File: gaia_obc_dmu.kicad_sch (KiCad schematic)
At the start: 7 parts, among them J2 Micro_SD_Card_Det2, U7 WLR089U0-I_RM

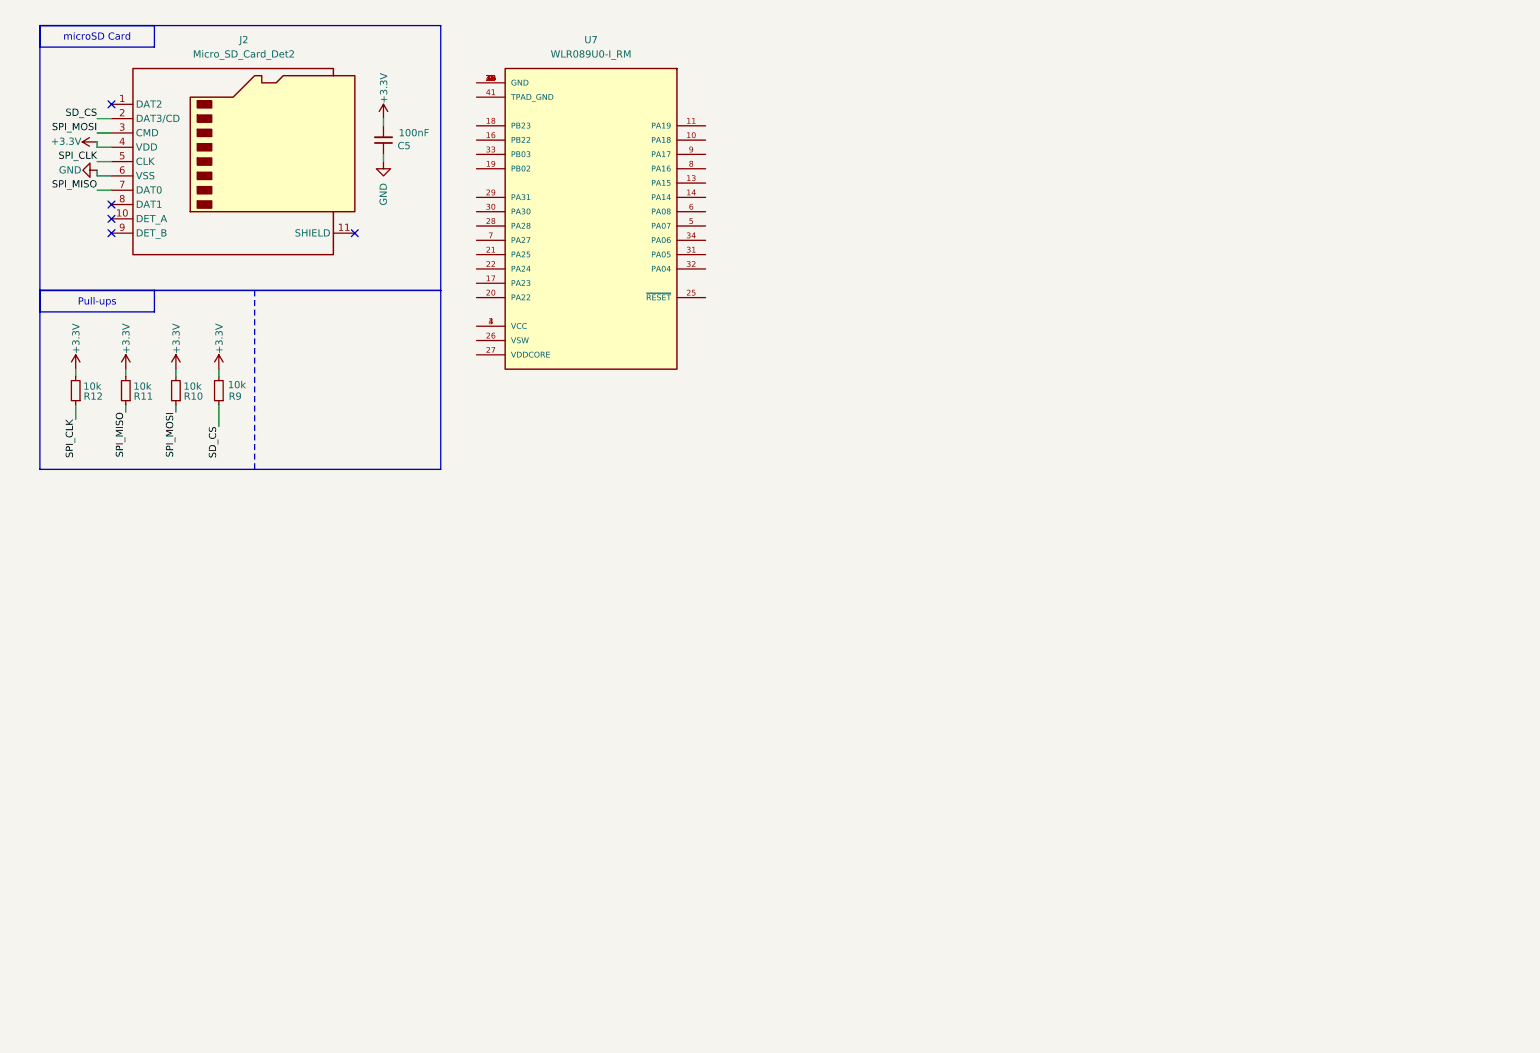
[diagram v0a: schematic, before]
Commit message: almost final release
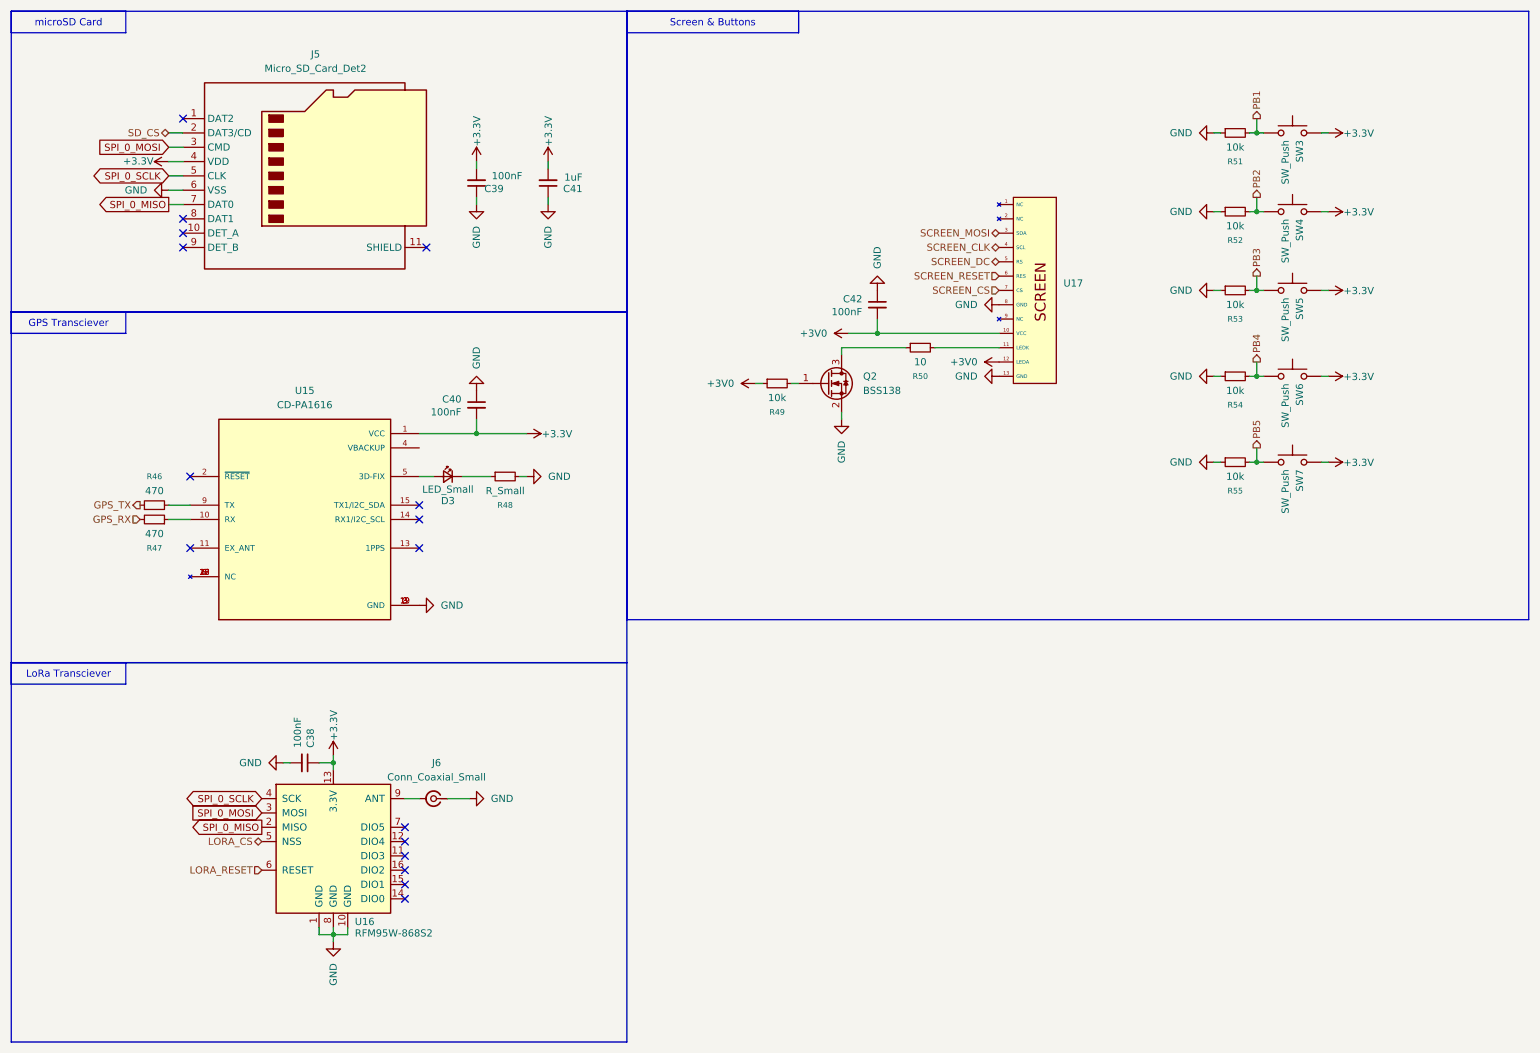
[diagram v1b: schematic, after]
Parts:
- removed R10, R11, R12, R9: 10k, symbol Device:R_Small
- removed U7: WLR089U0-I_RM, OnionSAT_Gaia:MODULE_WLR089U0-I_RM, symbol cs25_onionsat:WLR089U0-I_RM
- added C38, C40, C42: 100nF, Capacitor_SMD:C_0402_1005Metric, symbol Device:C_Small
- added C41: 1uF, Capacitor_SMD:C_0402_1005Metric, symbol Device:C_Small
- added D3: LED_Small, symbol Device:LED_Small
- added J6: Conn_Coaxial_Small, Connector_Coaxial:SMA_Amphenol_132134-10_Vertical, symbol Connector:Conn_Coaxial_Small
- added Q2: BSS138, Package_TO_SOT_SMD:SOT-23, symbol Transistor_FET:BSS138
- added R46, R47: 470, symbol Device:R_Small
- added R48: R_Small, symbol Device:R_Small
- added R49, R51, R52, R53, R54, R55: 10k, symbol Device:R_Small
- added R50: 10, symbol Device:R_Small
- added SW3, SW4, SW5, SW6, SW7: SW_Push, symbol Switch:SW_Push
- added U15: CD-PA1616, gaia_obc-footprints:XCVR_CD-PA1616D, symbol gaia_obc-symbols:CD-PA1616
- added U16: RFM95W-868S2, RF_Module:HOPERF_RFM9XW_SMD, symbol RF_Module:RFM95W-868S2
- added U17: ~, symbol gaia_obc-symbols:kepernyo
- C39: renamed from C5; footprint (none) -> Capacitor_SMD:C_0402_1005Metric
- renumbered J2 to J5
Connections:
- net +3.3V: now also C38.1, C40.2, C41.2, SW3.2, SW4.2, SW5.2, SW6.2, SW7.2, U15.1 (VCC), U16.13 (3.3V)
- net GND: now also C38.2, C40.1, C41.1, C42.1, J6.1 (In), Q2.2 (S), R48.2, R51.1, R52.1, R53.1, R54.1, R55.1, U15.12 (GND), U15.19 (GND), U15.3 (GND), U15.8 (GND), U16.1 (GND), U16.10 (GND), U16.8 (GND), U17.13 (GND), U17.8 (GND)
- net SPI_CLK renamed SPI_0_SCLK
- net SPI_0_SCLK: now also U16.4 (SCK)
- net SPI_MISO renamed SPI_0_MISO
- net SPI_0_MISO: now also U16.2 (MISO)
- net SPI_MOSI renamed SPI_0_MOSI
- net SPI_0_MOSI: now also U16.3 (MOSI)
- new net: J6.2 (Ext), U16.9 (ANT)
- new net: R47.1, U15.10 (RX)
- new net: U15.16 (NC), U15.17 (NC), U15.18 (NC), U15.20 (NC), U15.6 (NC), U15.7 (NC)
- new net: D3.2 (A), U15.5 (3D-FIX)
- new net: R46.2, U15.9 (TX)
- new net: Q2.3 (D), R50.1
- new net: R50.2, U17.11 (LEDK)
- new net: D3.1 (K), R48.1
- new net: Q2.1 (G), R49.2
- new net +3V0: C42.2, R49.1, U17.10 (VCC), U17.12 (LEDA)
- new net GPS_RX: R47.2
- new net GPS_TX: R46.1
- new net LORA_CS: U16.5 (NSS)
- new net LORA_RESET: U16.6 (RESET)
- new net PB1: R51.2, SW3.1
- new net PB2: R52.2, SW4.1
- new net PB3: R53.2, SW5.1
- new net PB4: R54.2, SW6.1
- new net PB5: R55.2, SW7.1
- new net SCREEN_CLK: U17.4 (SCL)
- new net SCREEN_CS: U17.7 (CS)
- new net SCREEN_DC: U17.5 (RS)
- new net SCREEN_MOSI: U17.3 (SDA)
- new net SCREEN_RESET: U17.6 (RES)
- no-connect marks 5 -> 16
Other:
- moved on the sheet: C39, J5

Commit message: prep for routing 2/1
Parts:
- D3: footprint (none) -> LED_SMD:LED_0603_1608Metric
- SW3, SW4, SW5, SW6, SW7: footprint (none) -> Button_Switch_SMD:SW_SPST_PTS647_Sx50
- U17: footprint (none) -> gaia_obc-footprints:kepernyo
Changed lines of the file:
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@@
 			)
 		)
-		(property "Footprint" ""
+		(property "Footprint" "Button_Switch_SMD:SW_SPST_PTS647_Sx50"
 			(at 241.3 30.48 0)
 			(effects
@@
 			)
 		)
-		(property "Footprint" ""
+		(property "Footprint" "Button_Switch_SMD:SW_SPST_PTS647_Sx50"
 			(at 241.3 44.45 0)
 			(effects
@@
 			)
 		)
-		(property "Footprint" ""
+		(property "Footprint" "Button_Switch_SMD:SW_SPST_PTS647_Sx50"
 			(at 241.3 58.42 0)
 			(effects
@@
 			)
 		)
-		(property "Footprint" ""
+		(property "Footprint" "LED_SMD:LED_0603_1608Metric"
 			(at 91.44 96.52 90)
 			(effects
@@
 			)
 		)
-		(property "Footprint" ""
+		(property "Footprint" "Button_Switch_SMD:SW_SPST_PTS647_Sx50"
 			(at 241.3 73.66 0)
 			(effects
@@
 			)
 		)
-		(property "Footprint" ""
+		(property "Footprint" "gaia_obc-footprints:kepernyo"
 			(at 199.39 46.99 0)
 			(effects
@@
 			)
 		)
-		(property "Footprint" ""
+		(property "Footprint" "Button_Switch_SMD:SW_SPST_PTS647_Sx50"
 			(at 241.3 88.9 0)
 			(effects
